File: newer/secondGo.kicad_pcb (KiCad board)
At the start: 2 copper layers, 115.6 x 119.4 mm, 67 parts, among them Q1 IRLZ34N, Q2 IRLZ34N, Q3 IRLZ34N, Q4 IRLZ34N, Q5 IRLZ34N, Q6 IRLZ34N, Q7 IRLZ34N, Q8 IRLZ34N, U1 Teensy3.5, U10 HCPL3120, U2 HCPL3120, U4 HCPL3120, U5 HCPL3120, U6 HCPL3120, U7 HCPL3120, U8 HCPL3120, U9 HCPL3120

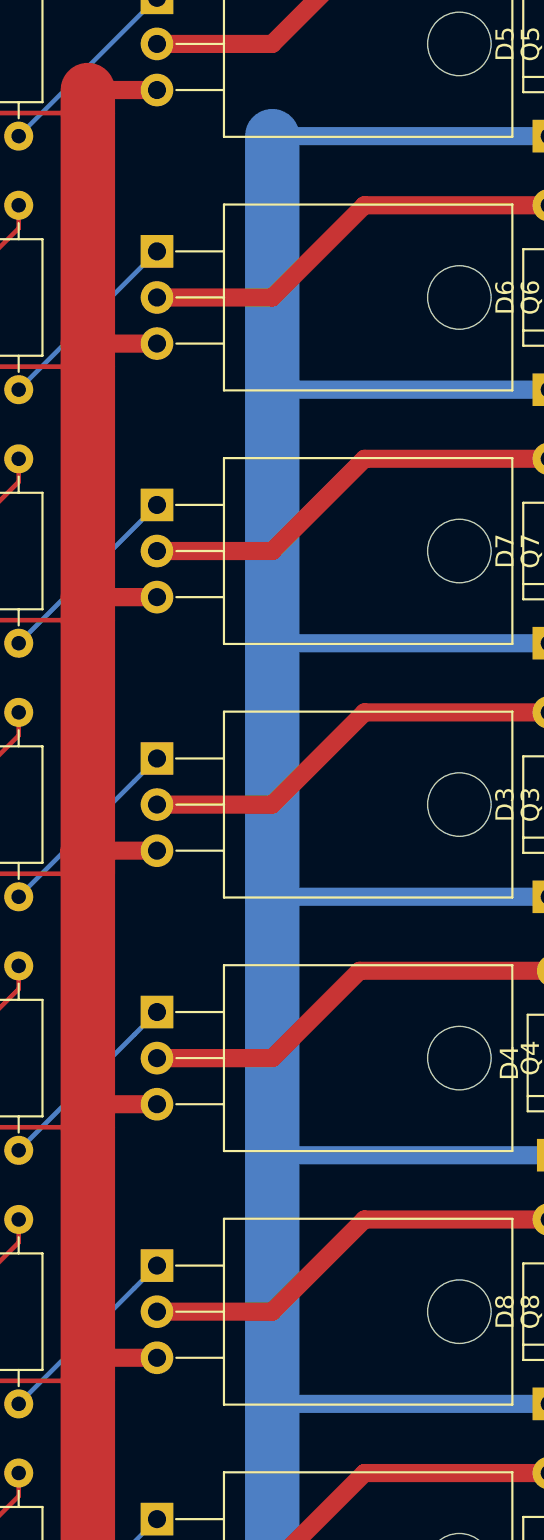
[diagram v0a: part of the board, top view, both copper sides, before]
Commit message: more updates
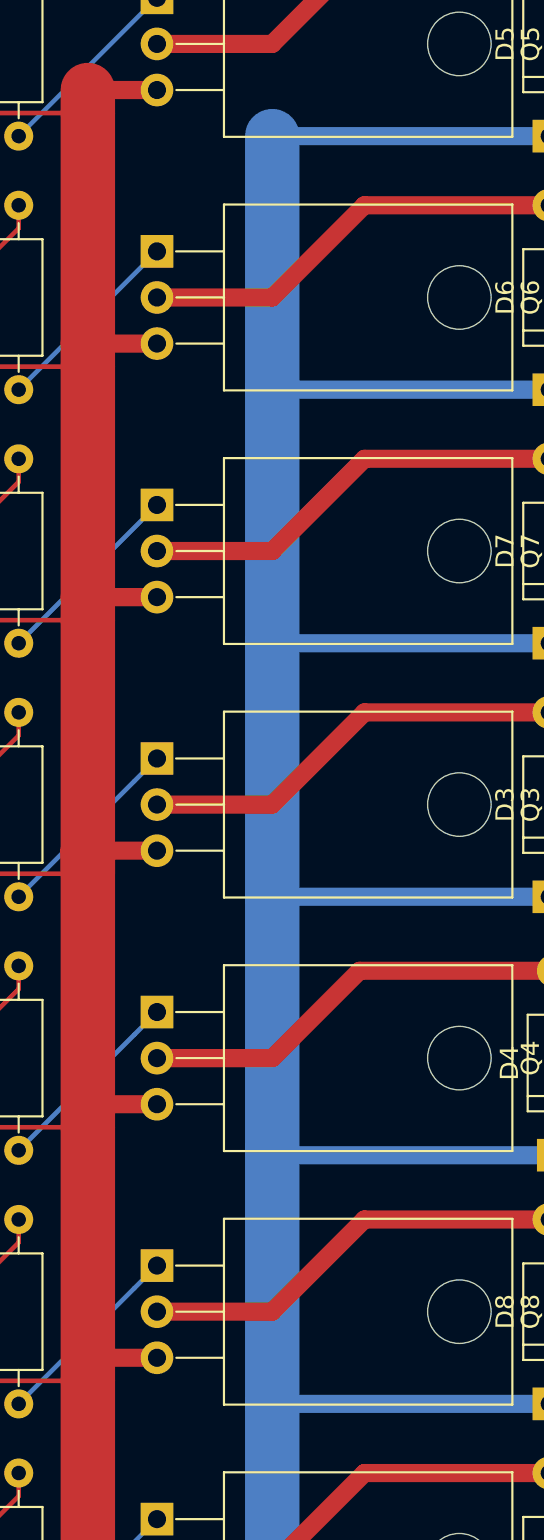
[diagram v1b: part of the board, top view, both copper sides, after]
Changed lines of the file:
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@@
   (general
     (links 157)
-    (no_connects 6)
-    (area 0 0 0 0)
+    (no_connects 5)
+    (area 170.930999 92.659999 288.340001 214.489)
     (thickness 1.6)
     (drawings 8)
-    (tracks 437)
+    (tracks 440)
     (zones 0)
     (modules 67)
@@
   (segment (start 246.38 123.19) (end 246.38 124.46) (width 0.254) (layer F.Cu) (net 7))
   (segment (start 246.38 124.46) (end 243.84 127) (width 0.254) (layer F.Cu) (net 7))
+  (segment (start 260.35 133.35) (end 260.35 119.38) (width 3) (layer B.Cu) (net 8))
+  (segment (start 260.35 119.38) (end 260.35 105.41) (width 3) (layer B.Cu) (net 8))
+  (segment (start 275.59 119.38) (end 260.35 119.38) (width 1) (layer B.Cu) (net 8))
+  (segment (start 260.35 175.26) (end 260.35 161.29) (width 3) (layer B.Cu) (net 8))
+  (segment (start 260.35 161.29) (end 260.35 147.32) (width 3) (layer B.Cu) (net 8))
+  (segment (start 275.834344 161.559448) (end 260.619448 161.559448) (width 1) (layer B.Cu) (net 8))
+  (segment (start 260.619448 161.559448) (end 260.35 161.29) (width 0.254) (layer B.Cu) (net 8))
   (segment (start 245.11 194.31) (end 245.11 205.74) (width 0.254) (layer B.Cu) (net 8))
   (segment (start 275.59 203.2) (end 260.35 203.2) (width 1) (layer B.Cu) (net 8))
@@
   (segment (start 260.35 189.23) (end 260.35 175.26) (width 3) (layer B.Cu) (net 8))
   (segment (start 275.59 189.23) (end 260.35 189.23) (width 1) (layer B.Cu) (net 8))
-  (segment (start 260.35 175.26) (end 260.35 147.32) (width 3) (layer B.Cu) (net 8))
   (segment (start 275.59 175.26) (end 260.35 175.26) (width 1) (layer B.Cu) (net 8))
-  (segment (start 275.834344 161.559448) (end 260.619448 161.559448) (width 1) (layer B.Cu) (net 8))
   (segment (start 260.35 147.32) (end 260.35 133.35) (width 3) (layer B.Cu) (net 8))
   (segment (start 275.59 147.32) (end 260.35 147.32) (width 1) (layer B.Cu) (net 8))
-  (segment (start 260.35 133.35) (end 260.35 105.41) (width 3) (layer B.Cu) (net 8))
   (segment (start 275.59 133.35) (end 260.35 133.35) (width 1) (layer B.Cu) (net 8))
-  (segment (start 275.59 119.38) (end 260.35 119.38) (width 1) (layer B.Cu) (net 8))
   (segment (start 260.35 105.41) (end 275.59 105.41) (width 1) (layer B.Cu) (net 8))
   (segment (start 250.220078 205.74) (end 260.35 205.74) (width 3) (layer B.Cu) (net 8))
